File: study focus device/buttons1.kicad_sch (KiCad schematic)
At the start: 17 parts, among them U1 MCP23017_SP

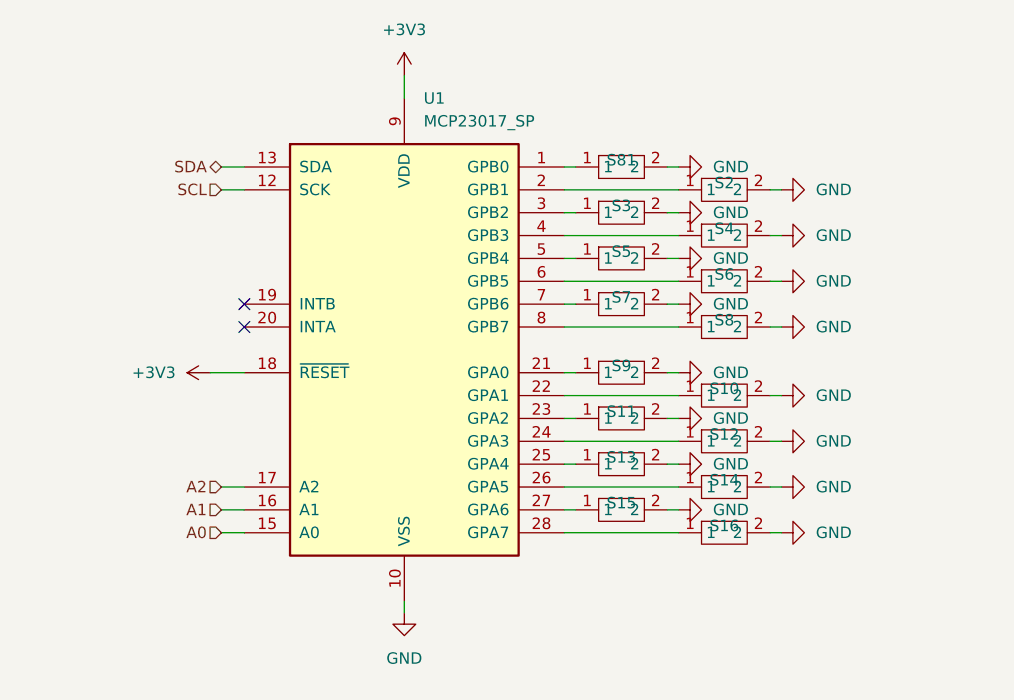
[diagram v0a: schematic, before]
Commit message: more work
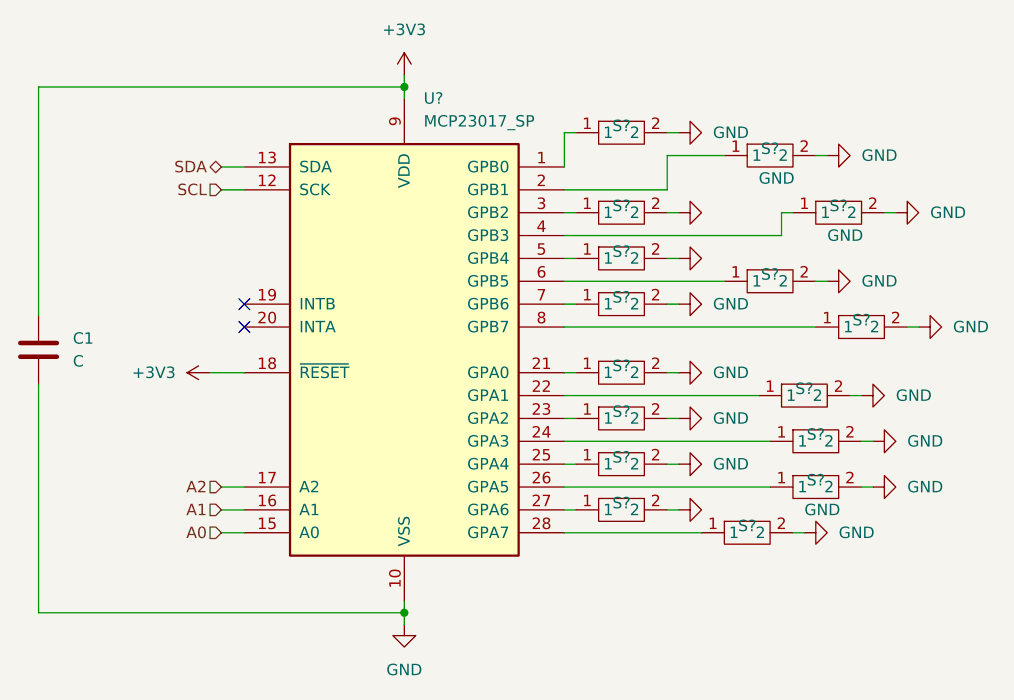
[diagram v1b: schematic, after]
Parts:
- added C1: C, Capacitor_THT:C_Radial_D5.0mm_H11.0mm_P2.00mm, symbol Device:C
- renumbered S81 to S?, S15 to S?, S13 to S?, S8 to S?, S6 to S?, S10 to S?, S12 to S?, S7 to S?, S11 to S?, S14 to S?, S5 to S?, S4 to S?, S16 to S?, S3 to S?, S9 to S?, S2 to S?, U1 to U?
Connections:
- net +3V3: now also C1.1
- net GND: now also C1.2
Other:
- moved on the sheet: S?
